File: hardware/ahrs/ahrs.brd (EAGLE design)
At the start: 21 x 40 mm, 32 parts, among them J1 2-PIN, U1 LSM9DS1, U2 STM32G4_UFQFPN48_T1, X1 NX2016SA24MHZ-EXS00A-CS11335, X2 SM08B-SRSS-TB

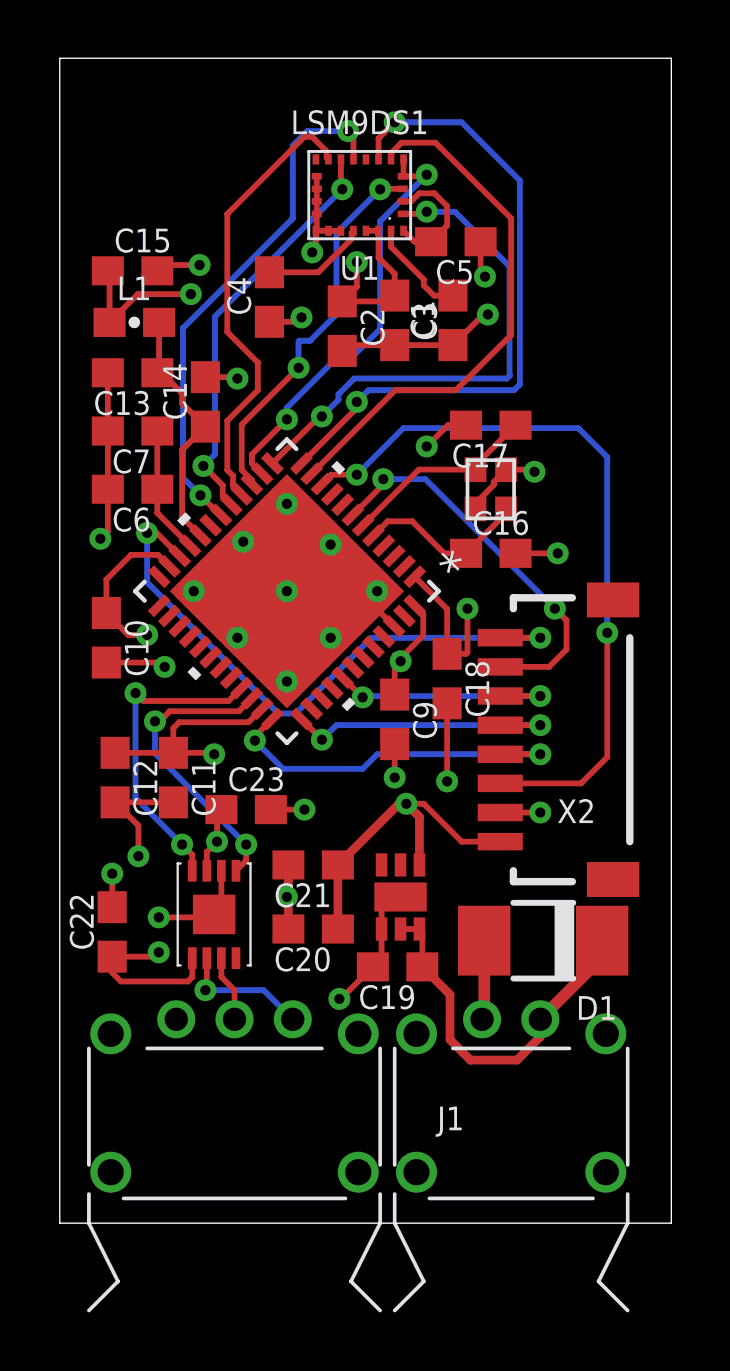
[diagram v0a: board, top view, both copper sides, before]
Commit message: Prior to pulling from fusion
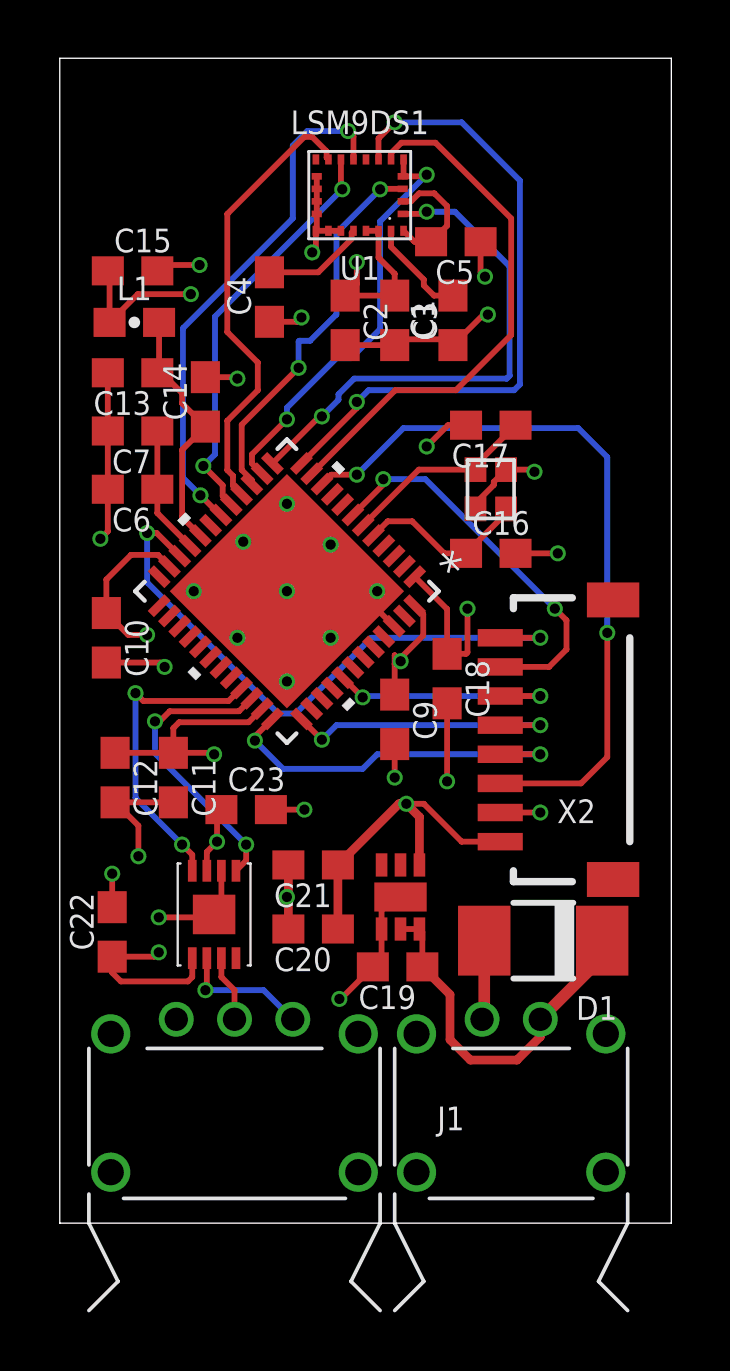
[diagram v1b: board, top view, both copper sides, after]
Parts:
- C1, C2, C3, C4, C5: device timlib:C0603 -> rcl:C0603
- X2: device con-jst2:SM08B-SRSS-TB -> timlib:SM08B-SRSS-TB
- moved C2 0.22 mm to (9.80, 31.0)
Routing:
- net GND: vias 27 -> 28
